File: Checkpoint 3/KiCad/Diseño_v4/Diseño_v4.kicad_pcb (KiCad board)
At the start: 2 copper layers, 145 x 95 mm, 51 parts, among them J1 Conn_01x02, J2 Conn_01x02, Q1 BC547, Q2 BC547, Q3 BC557, Q4 BC557, Q5 BC547, Q6 TIP32A, Q7 BC547, Q8 BC547, Q9 BC547, U1 TL431LP, U2 LM358

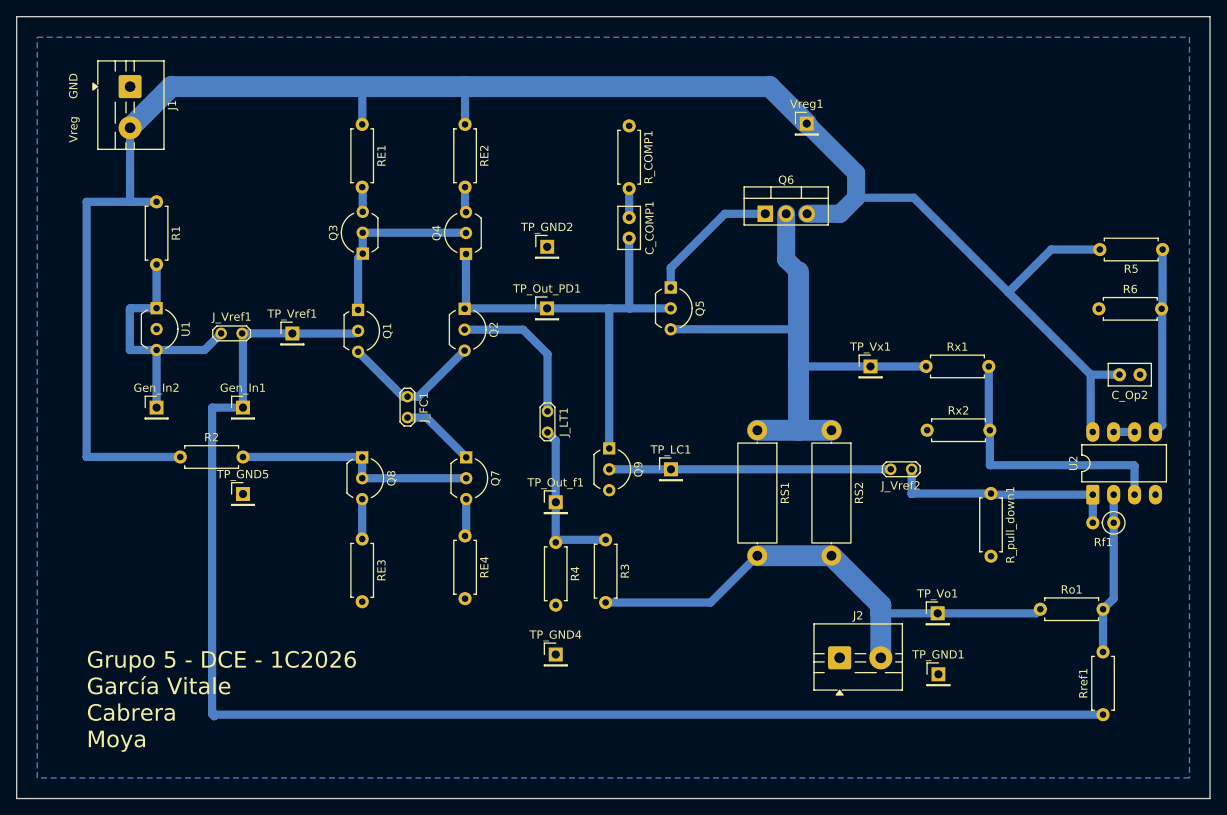
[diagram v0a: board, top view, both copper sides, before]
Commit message: corrección pcb
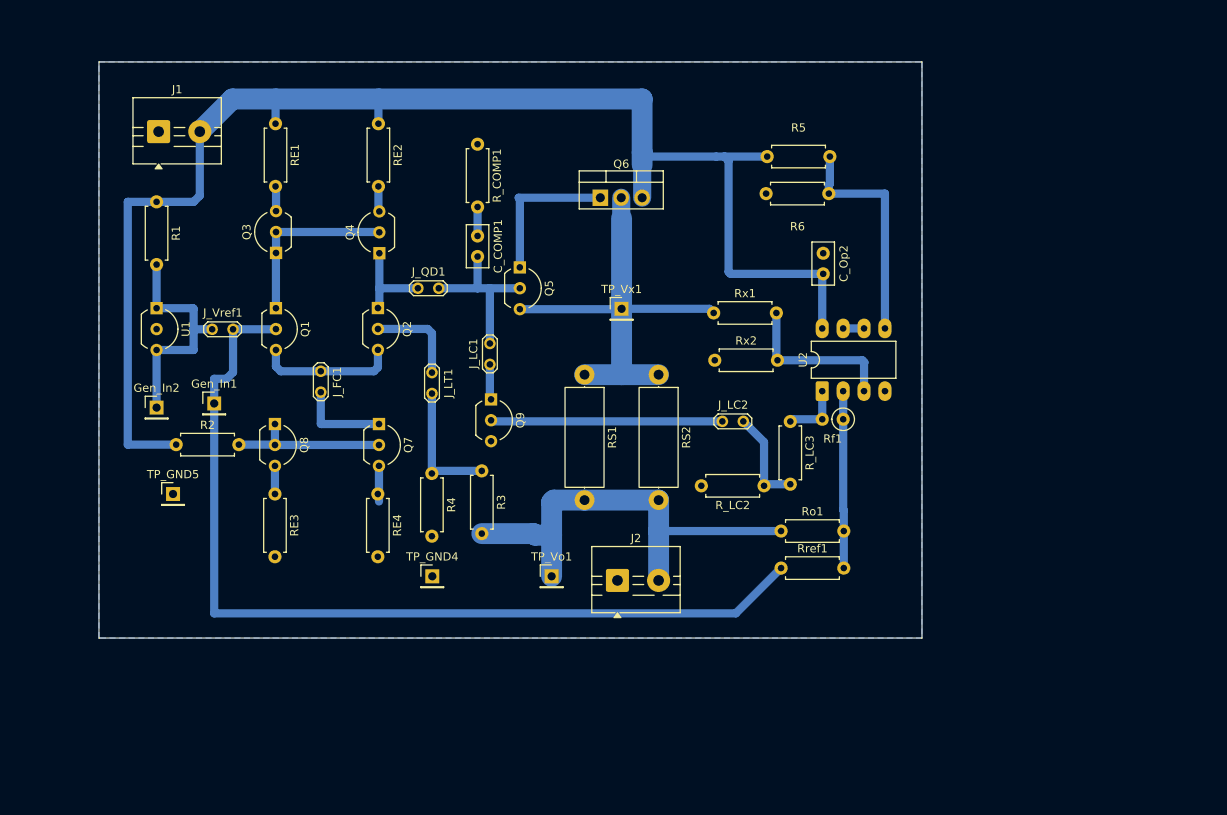
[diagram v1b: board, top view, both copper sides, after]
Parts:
- removed TP_GND1, TP_GND2, TP_LC1, TP_Out_PD1, TP_Out_f1, TP_Vref1, Vreg1: ~, Connector_PinHeader_2.54mm:PinHeader_1x01_P2.54mm_Vertical
- added J_LC2: ~, TestPoint:TestPoint_2Pads_Pitch2.54mm_Drill0.8mm, F.Cu at (153.2, 76.7)
- added J_QD1: ~, TestPoint:TestPoint_2Pads_Pitch2.54mm_Drill0.8mm, F.Cu at (116.2, 60.5)
- added R_LC3: 3k9, Resistor_THT:R_Axial_DIN0207_L6.3mm_D2.5mm_P7.62mm_Horizontal, F.Cu at (161.5, 76.7)
- R_LC2: renamed from R_pull_down1; value R -> 1k
- moved J_LC1 52.8 mm to (125.0, 69.8), turned to 90 degrees
- moved TP_Vo1 47.1 mm to (132.5, 95.5)
- moved Rref1 43.0 mm to (160.4, 94.5), turned to 0 degrees
- moved R6 42.8 mm to (158.6, 49.0)
- moved R5 42.0 mm to (166.3, 44.5)
- moved C_Op2 41.2 mm to (165.5, 56.2), turned to -90 degrees
- moved U2 35.2 mm to (165.4, 73.0)
- moved Rf1 35.2 mm to (167.9, 76.4)
- moved Ro1 32.9 mm to (160.4, 90.0)
- moved TP_Vx1 31.0 mm to (141.0, 63.0)
- moved J2 28.6 mm to (140.5, 96.0)
- moved R_LC2 27.6 mm to (158.3, 84.5), turned to 180 degrees
- moved Rx2 27.2 mm to (152.3, 69.2)
- moved Rx1 26.6 mm to (152.2, 63.5)
- moved RS1 22.1 mm to (136.5, 71.0)
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- renumbered J_Vref2 to J_LC1
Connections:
- C_COMP1 pad 2: Net-(Q2-C) -> Net-(J_LC1-B)
- J_LC1 pad 1: Net-(J_Vref2-A) -> Net-(J_LC1-A)
- J_LC1 pad 2: /Vf -> Net-(J_LC1-B)
- Q2 pad 1: Net-(Q2-C) -> Net-(J_QD1-A)
- Q4 pad 1: Net-(Q2-C) -> Net-(J_QD1-A)
- Q5 pad 2: Net-(Q2-C) -> Net-(J_LC1-B)
- Q9 pad 1: Net-(Q2-C) -> Net-(J_LC1-A)
- R_LC2 pad 1: Net-(J_Vref2-A) -> Net-(J_LC2-B)
- Rf1 pad 2: Net-(J_Vref2-A) -> Net-(R_LC3-Pad1)
- U2 pad 1: Net-(J_Vref2-A) -> Net-(R_LC3-Pad1)
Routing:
- net /Vreg: track 234.3 -> 173.6 mm
- net /Vref: track 172.1 -> 112.7 mm
- net Net-(Q2-C): track 57.1 -> 0.00 mm
- net Net-(J_Vref2-A): track 28.5 -> 0.00 mm
- net Net-(J_LC1-B): track 0.00 -> 20.4 mm
- net Net-(U2A-+): track 33.2 -> 20.0 mm
- net /Vx: track 67.2 -> 54.3 mm
- net Net-(J_LC2-B): track 0.00 -> 12.1 mm
- net Net-(J_QD1-A): track 0.00 -> 11.2 mm
- net Net-(Q7-B): track 29.7 -> 19.6 mm
- net /Vo: track 64.3 -> 55.3 mm
- net Net-(R_LC3-Pad1): track 0.00 -> 7.41 mm
- net Net-(J_LT1-A): track 18.3 -> 11.6 mm
- net /Vf: track 34.2 -> 28.2 mm
- net Net-(U2B-+): track 22.3 -> 27.8 mm
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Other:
- board size 145 x 95 mm -> 100 x 70 mm
- board text removed: "GND"
- board text removed: "Grupo 5 - DCE - 1C2026 García Vitale Cabrera Moya"
- board text removed: "Vreg"
